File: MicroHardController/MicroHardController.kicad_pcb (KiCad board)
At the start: 2 copper layers, 135.5 x 143.5 mm, 2 parts, among them U1 THB001P

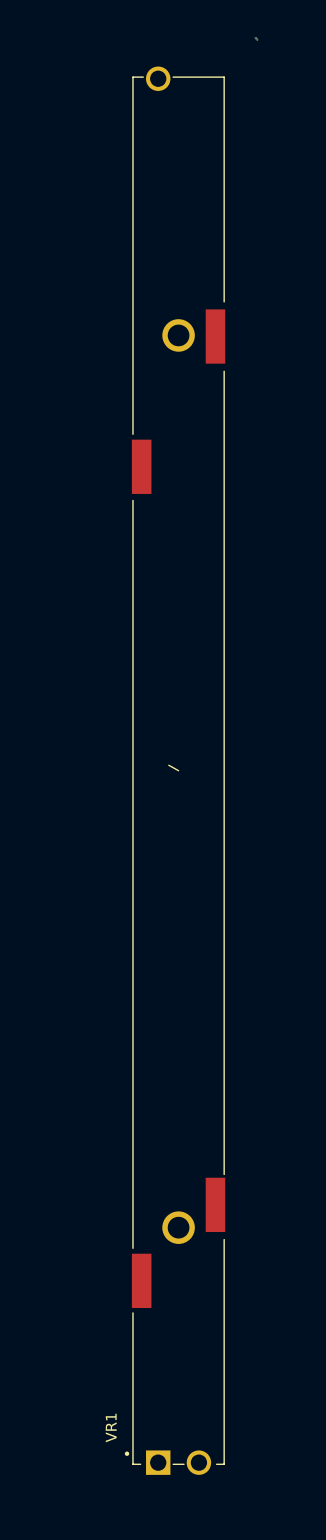
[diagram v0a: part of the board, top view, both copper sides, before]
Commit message: IDK what this commit does, best to ignore it tb tbj
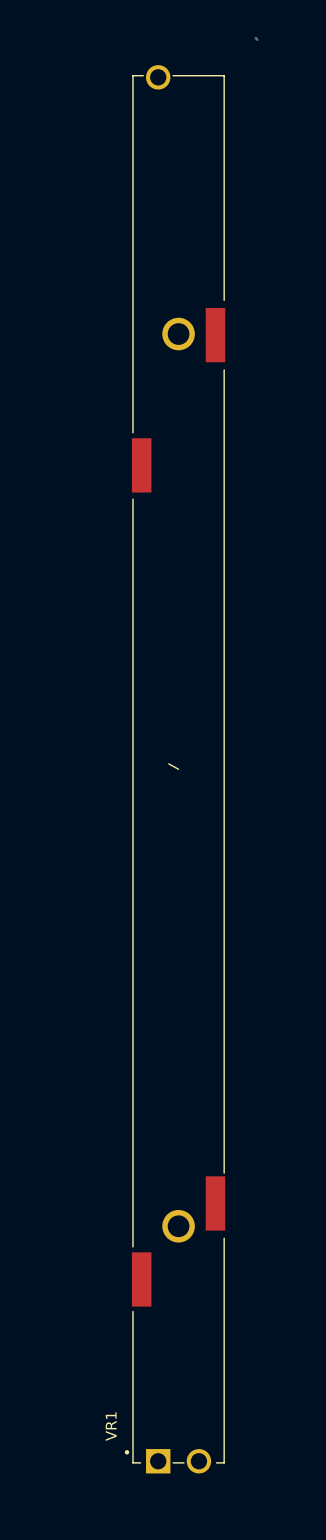
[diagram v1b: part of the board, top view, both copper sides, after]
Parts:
- moved VR1 0.13 mm to (63.9, 71.9)
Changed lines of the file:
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@@
 	(footprint "MicroHard:TRIM_PS100-1B1BR10K"
 		(layer "F.Cu")
-		(at 63.9 72 90)
+		(at 63.9 71.87 90)
 		(property "Reference" "VR1"
 			(at -60.505 -6.17 90)
